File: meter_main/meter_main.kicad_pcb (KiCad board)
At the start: 2 copper layers, 33 x 32 mm, 22 parts, among them J1 ADC, J2 USB_CDC, J3 HOST_PROG, Q1 S8050, U1 ESP32-S3-WROOM-1, U2 AMS1117/WL9005P3

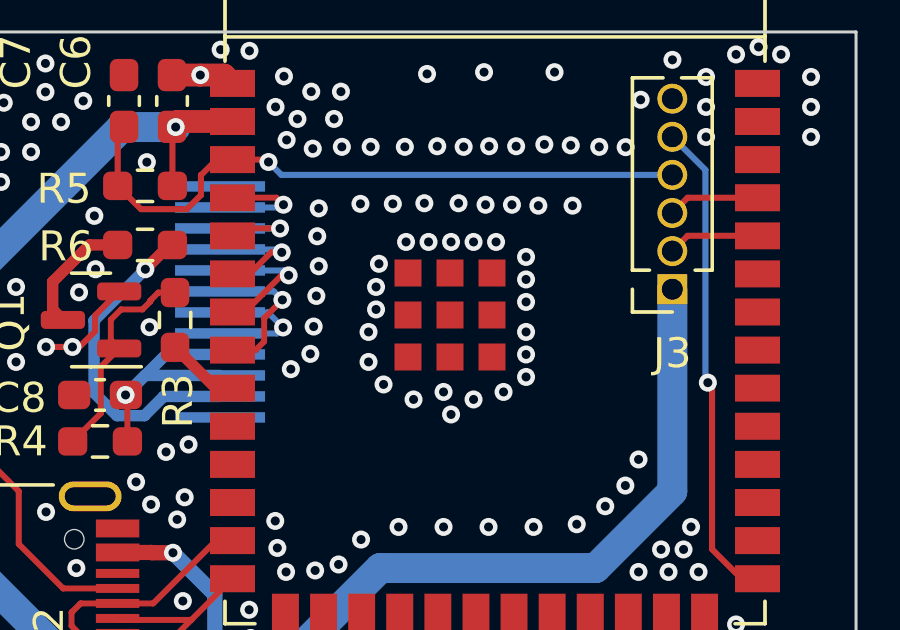
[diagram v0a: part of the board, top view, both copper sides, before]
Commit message: Generate Rev. 1 gerber
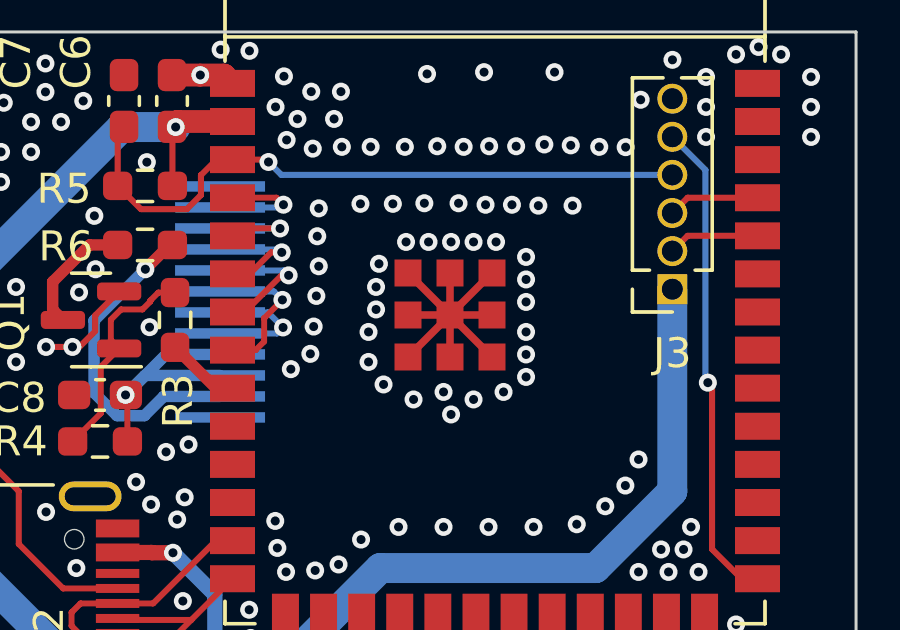
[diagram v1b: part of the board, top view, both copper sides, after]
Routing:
- net GND: track 12.6 -> 26.1 mm
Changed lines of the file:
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@@
   (segment (start 92.9375 89.4375) (end 93.215 89.715) (width 0.762) (layer "F.Cu") (net 2))
   (segment (start 96.4 113.3875) (end 98.5375 113.3875) (width 0.762) (layer "F.Cu") (net 2))
+  (segment (start 101.865 96.035) (end 99.065 98.835) (width 0.25) (layer "F.Cu") (net 2))
+  (segment (start 101.865 97.435) (end 100.465 97.435) (width 0.25) (layer "F.Cu") (net 2))
   (segment (start 88.63567 97.45183) (end 88.63567 97.975671) (width 0.2032) (layer "F.Cu") (net 2))
   (segment (start 89.4375 96.65) (end 88.63567 97.45183) (width 0.2032) (layer "F.Cu") (net 2))
@@
   (segment (start 92.1425 89.4375) (end 92.9375 89.4375) (width 0.762) (layer "F.Cu") (net 2))
   (segment (start 98.5375 113.3875) (end 98.75 113.6) (width 0.762) (layer "F.Cu") (net 2))
+  (segment (start 99.065 97.435) (end 100.465 97.435) (width 0.25) (layer "F.Cu") (net 2))
   (segment (start 87.88 98.5) (end 87 98.5) (width 0.2032) (layer "F.Cu") (net 2))
+  (segment (start 101.865 98.835) (end 99.065 96.035) (width 0.25) (layer "F.Cu") (net 2))
+  (segment (start 100.465 97.435) (end 100.465 98.835) (width 0.25) (layer "F.Cu") (net 2))
+  (segment (start 100.465 96.035) (end 100.465 97.435) (width 0.25) (layer "F.Cu") (net 2))
   (via (at 104.75 117.75) (size 0.6) (drill 0.3) (layers "F.Cu" "B.Cu") (free) (net 2))
   (via (at 108.75 106) (size 0.6) (drill 0.3) (layers "F.Cu" "B.Cu") (free) (net 2))
